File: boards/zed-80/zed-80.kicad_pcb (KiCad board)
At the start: 2 copper layers, 99.5 x 70 mm, 34 parts, among them J401 TYPE-C-31-M-12, SW201 SW_Push, U201 GD74LS04, U202 Z84C0010PEC, U301 TT74LS32BI, U302 AT28C256-15PU, U303 HM628128BLP-10, U401 CH340C, U402 MC68B50P, Y201 7.3728 MHz

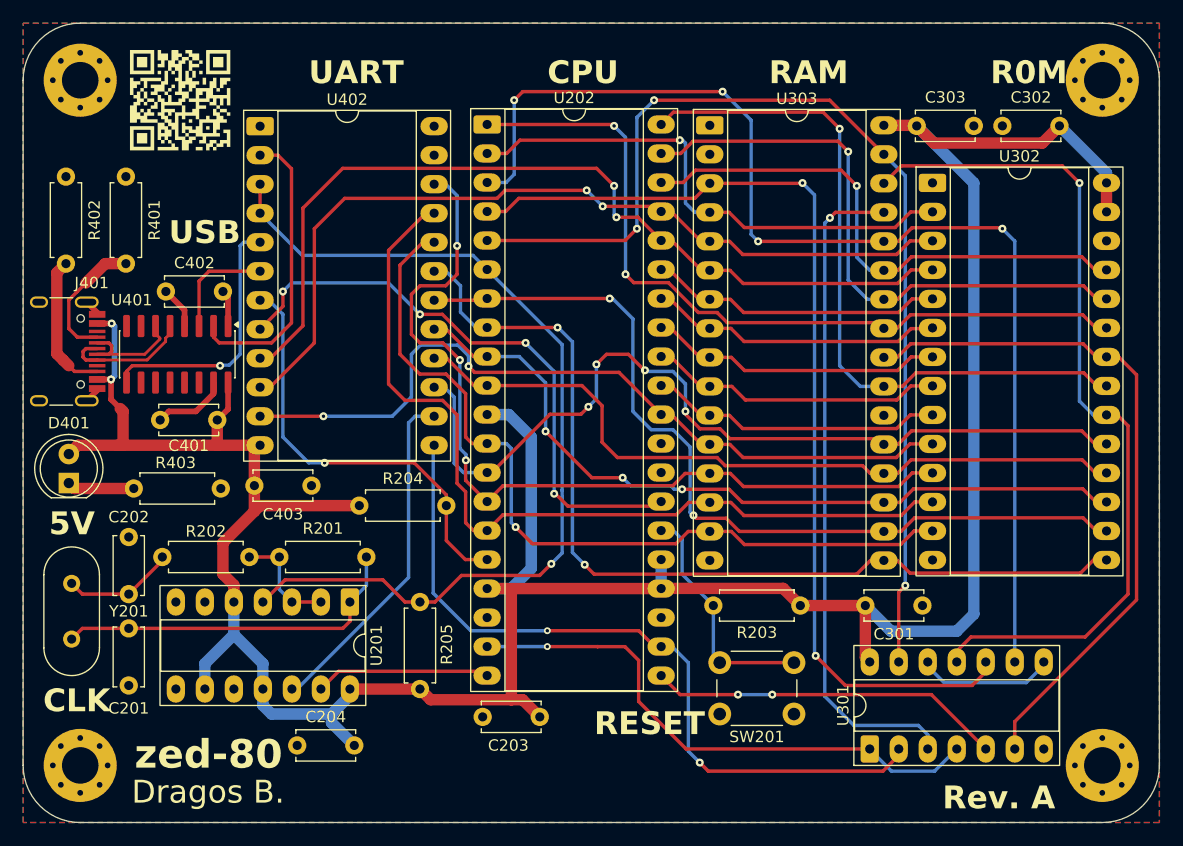
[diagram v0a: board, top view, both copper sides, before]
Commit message: Cleanup main board
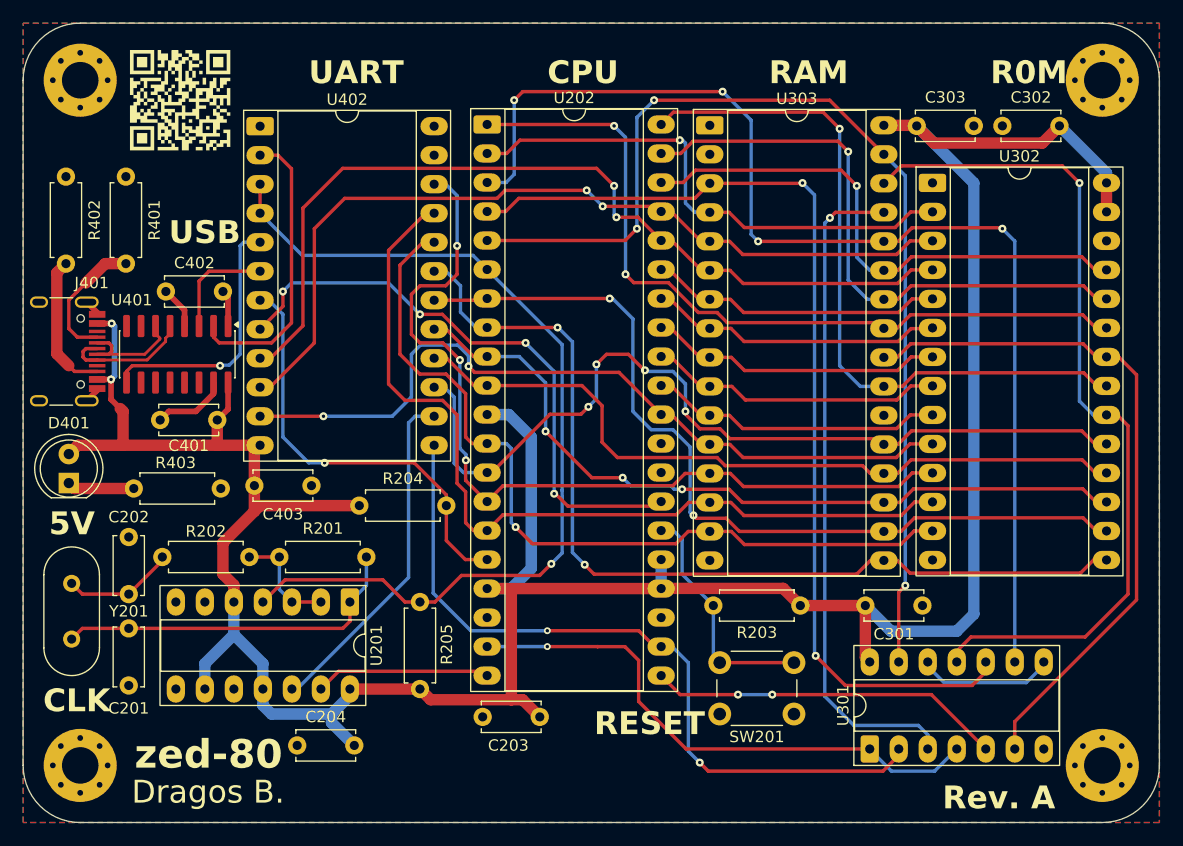
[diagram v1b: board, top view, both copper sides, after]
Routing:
- net /USB-to-UART/D-: track 10.6 -> 9.91 mm
- net /USB-to-UART/D+: track 11.4 -> 10.7 mm
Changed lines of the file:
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@@
-	)
-	(segment
-		(start 93.69 89.56)
-		(end 93.69 89.25)
-		(width 0.3)
-		(layer "F.Cu")
-		(net 3)
 	)
 	(segment
@@
 	)
 	(segment
-		(start 85.5 80.235)
-		(end 85.515 80.235)
-		(width 1)
-		(layer "F.Cu")
-		(net 4)
-	)
-	(segment
 		(start 89.25 68.8)
 		(end 87.985 68.8)
@@
 	)
 	(segment
-		(start 159.7 51.45)
-		(end 159.75 51.5)
-		(width 1)
-		(layer "F.Cu")
-		(net 4)
-	)
-	(segment
 		(start 125.24 101.75)
 		(end 124.25 101.75)
@@
 	(segment
 		(start 86.285 79.465)
-		(end 89.75 79.465)
-		(width 1)
-		(layer "F.Cu")
-		(net 4)
-	)
-	(segment
-		(start 89.75 79.465)
 		(end 90.25 79.465)
 		(width 1)
@@
 	)
 	(segment
-		(start 94.365 69.025)
-		(end 94.365 69.7)
-		(width 0.25)
-		(layer "F.Cu")
-		(net 7)
-	)
-	(segment
 		(start 92.353554 72)
 		(end 87.985 72)
@@
 	)
 	(segment
-		(start 93.095 69.025)
-		(end 93.095 69.7)
-		(width 0.25)
-		(layer "F.Cu")
-		(net 8)
-	)
-	(segment
 		(start 89 70.5)
 		(end 89.25 70.75)
@@
 	(segment
 		(start 84.450001 71.450001)
-		(end 85 72)
-		(width 1)
-		(layer "F.Cu")
-		(net 11)
-	)
-	(segment
-		(start 85 72)
 		(end 85.5 72.5)
 		(width 1)
@@
 	)
 	(segment
-		(start 85.5 66.75)
-		(end 85.5 66.746504)
-		(width 0.3)
-		(layer "F.Cu")
-		(net 12)
-	)
-	(segment
 		(start 88.69 63.56)
 		(end 87 65.25)
@@
 	(segment
 		(start 85.5 69.25)
-		(end 85.5 66.75)
-		(width 0.3)
-		(layer "F.Cu")
+		(end 85.5 66.746504)
+		(width 0.3)
+		(layer "F.Cu")
